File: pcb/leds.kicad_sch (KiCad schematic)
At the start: 55 parts

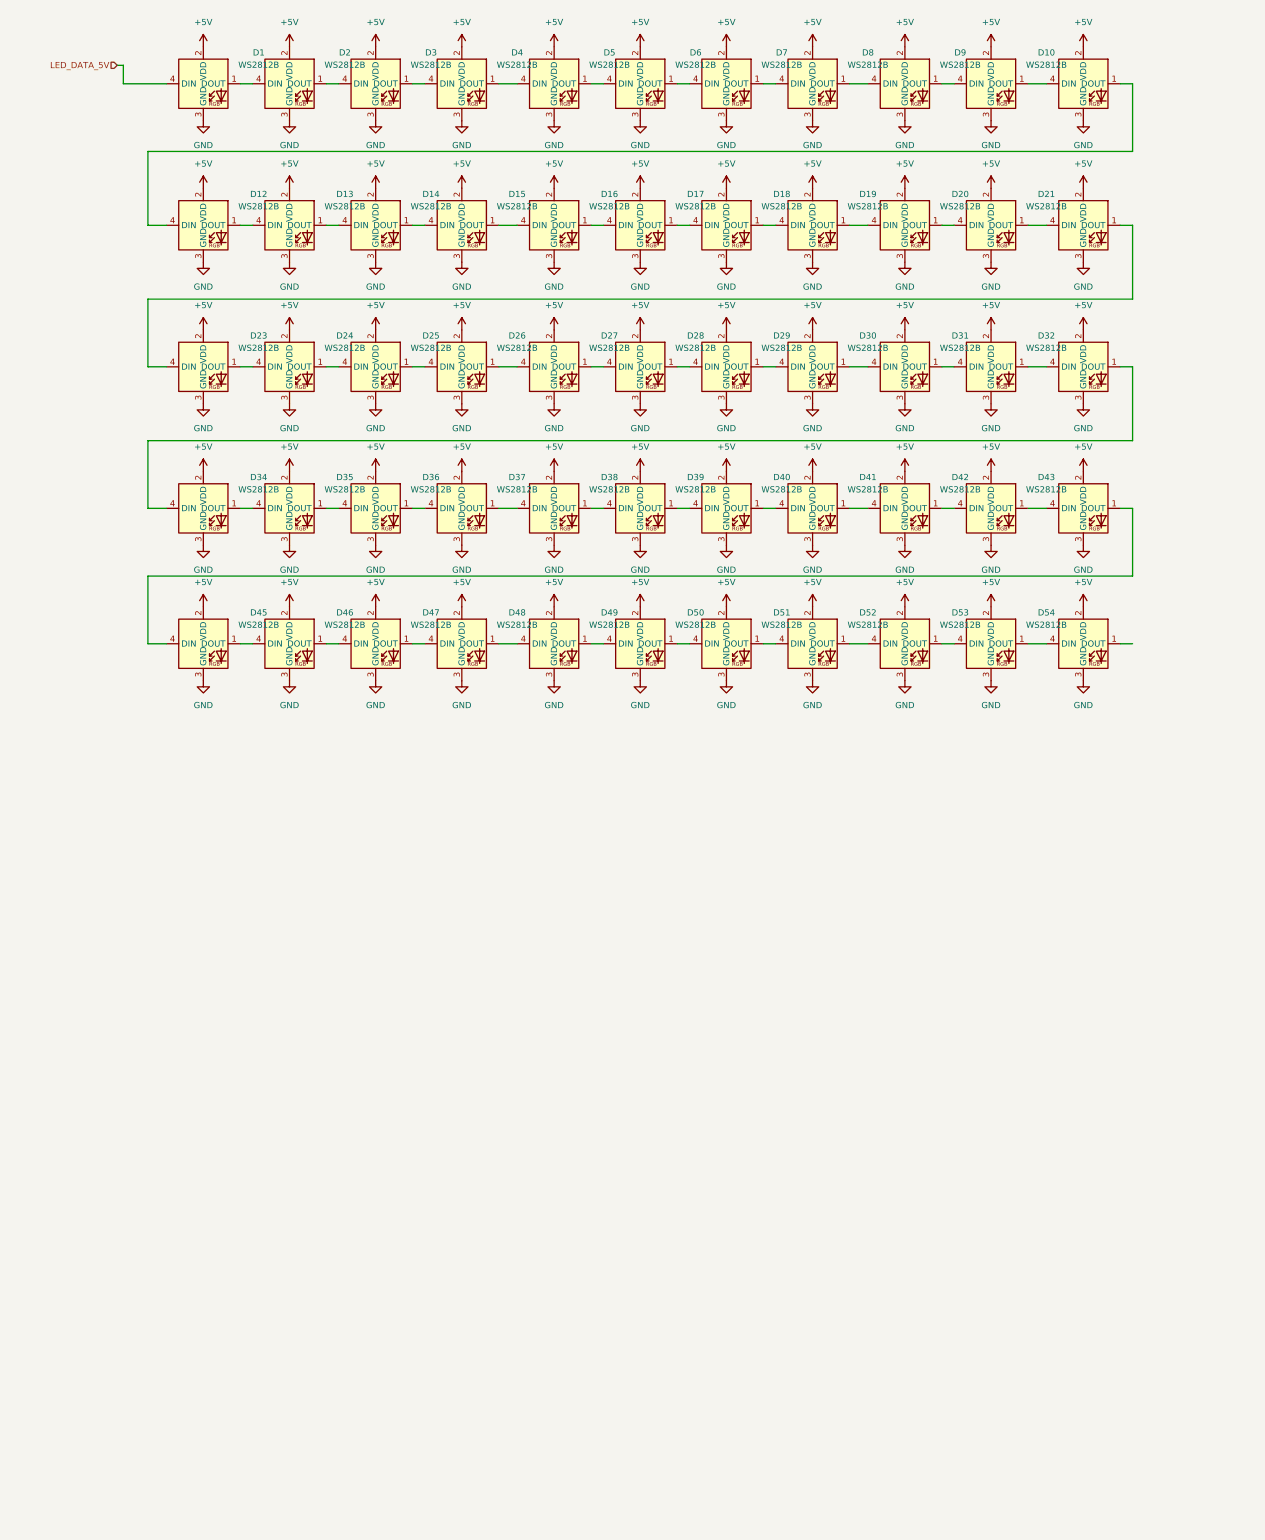
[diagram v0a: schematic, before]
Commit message: server updates and battling with kicad
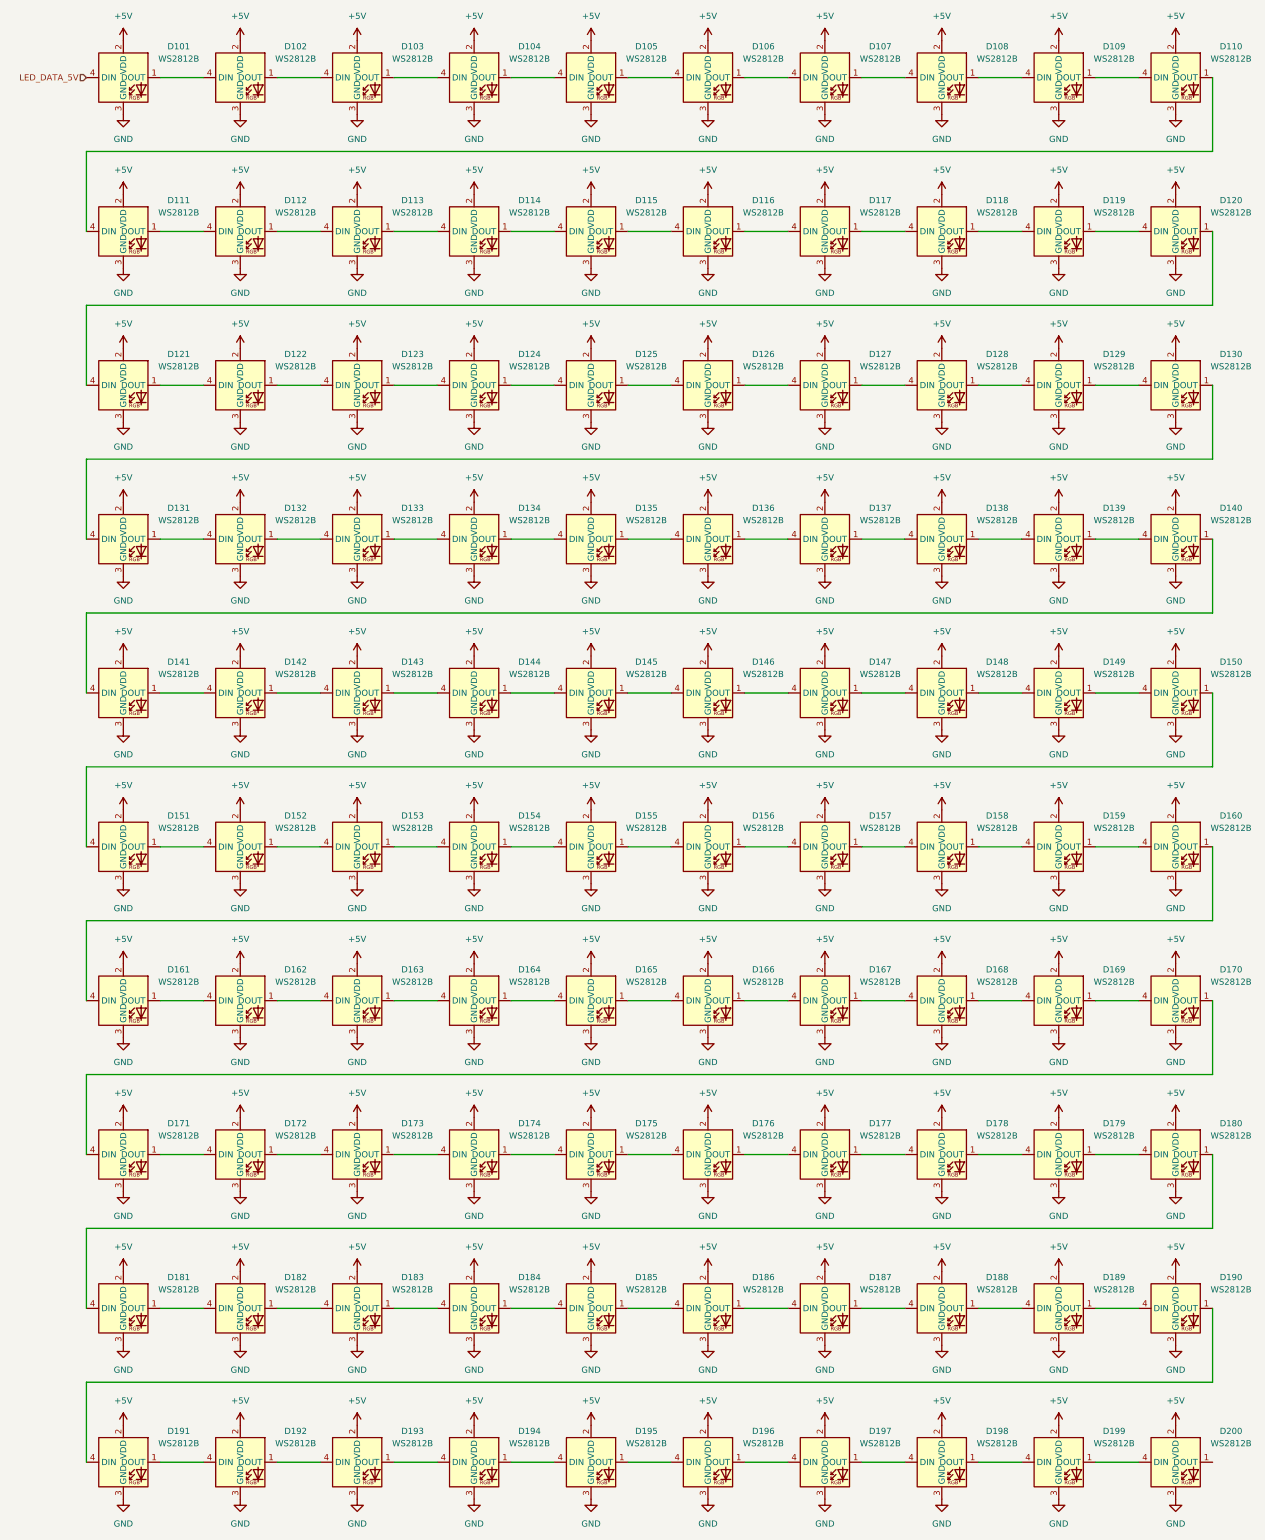
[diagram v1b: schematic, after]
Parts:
- removed D10, D11, D12, D13, D14, D15, D16, D17, D18, D19, D2, D20, D21, D22, D23, D24, D25, D26, D27, D28, D29, D3, D30, D31, D32, D33, D34, D35, D36, D37, D38, D39, D4, D40, D41, D42, D43, D44, D45, D46, D47, D48, D49, D5, D50, D51, D52, D53, D54, D55, D6, D7, D8, D9: WS2812B, PCM_JLCPCB:LED-SMD_4P-L1.6-W1.5_XL-1615RGBC-WS2812B, symbol PCM_JLCPCB-Extended:LED, WS2812B, 1615
- added D102, D103, D104, D105, D106, D107, D108, D109, D110, D111, D112, D113, D114, D115, D116, D117, D118, D119, D120, D121, D122, D123, D124, D125, D126, D127, D128, D129, D130, D131, D132, D133, D134, D135, D136, D137, D138, D139, D140, D141, D142, D143, D144, D145, D146, D147, D148, D149, D150, D151, D152, D153, D154, D155, D156, D157, D158, D159, D160, D161, D162, D163, D164, D165, D166, D167, D168, D169, D170, D171, D172, D173, D174, D175, D176, D177, D178, D179, D180, D181, D182, D183, D184, D185, D186, D187, D188, D189, D190, D191, D192, D193, D194, D195, D196, D197, D198, D199, D200: WS2812B, PCM_JLCPCB:LED-SMD_4P-L1.6-W1.5_XL-1615RGBC-WS2812B, symbol PCM_JLCPCB-Extended:LED, WS2812B, 1615
- renumbered D1 to D101
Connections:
- net +5V: now also D102.2 (VDD), D103.2 (VDD), D104.2 (VDD), D105.2 (VDD), D106.2 (VDD), D107.2 (VDD), D108.2 (VDD), D109.2 (VDD), D110.2 (VDD), D111.2 (VDD), D112.2 (VDD), D113.2 (VDD), D114.2 (VDD), D115.2 (VDD), D116.2 (VDD), D117.2 (VDD), D118.2 (VDD), D119.2 (VDD), D120.2 (VDD), D121.2 (VDD), D122.2 (VDD), D123.2 (VDD), D124.2 (VDD), D125.2 (VDD), D126.2 (VDD), D127.2 (VDD), D128.2 (VDD), D129.2 (VDD), D130.2 (VDD), D131.2 (VDD), D132.2 (VDD), D133.2 (VDD), D134.2 (VDD), D135.2 (VDD), D136.2 (VDD), D137.2 (VDD), D138.2 (VDD), D139.2 (VDD), D140.2 (VDD), D141.2 (VDD), D142.2 (VDD), D143.2 (VDD), D144.2 (VDD), D145.2 (VDD), D146.2 (VDD), D147.2 (VDD), D148.2 (VDD), D149.2 (VDD), D150.2 (VDD), D151.2 (VDD), D152.2 (VDD), D153.2 (VDD), D154.2 (VDD), D155.2 (VDD), D156.2 (VDD), D157.2 (VDD), D158.2 (VDD), D159.2 (VDD), D160.2 (VDD), D161.2 (VDD), D162.2 (VDD), D163.2 (VDD), D164.2 (VDD), D165.2 (VDD), D166.2 (VDD), D167.2 (VDD), D168.2 (VDD), D169.2 (VDD), D170.2 (VDD), D171.2 (VDD), D172.2 (VDD), D173.2 (VDD), D174.2 (VDD), D175.2 (VDD), D176.2 (VDD), D177.2 (VDD), D178.2 (VDD), D179.2 (VDD), D180.2 (VDD), D181.2 (VDD), D182.2 (VDD), D183.2 (VDD), D184.2 (VDD), D185.2 (VDD), D186.2 (VDD), D187.2 (VDD), D188.2 (VDD), D189.2 (VDD), D190.2 (VDD), D191.2 (VDD), D192.2 (VDD), D193.2 (VDD), D194.2 (VDD), D195.2 (VDD), D196.2 (VDD), D197.2 (VDD), D198.2 (VDD), D199.2 (VDD), D200.2 (VDD)
- net GND: now also D102.3 (GND), D103.3 (GND), D104.3 (GND), D105.3 (GND), D106.3 (GND), D107.3 (GND), D108.3 (GND), D109.3 (GND), D110.3 (GND), D111.3 (GND), D112.3 (GND), D113.3 (GND), D114.3 (GND), D115.3 (GND), D116.3 (GND), D117.3 (GND), D118.3 (GND), D119.3 (GND), D120.3 (GND), D121.3 (GND), D122.3 (GND), D123.3 (GND), D124.3 (GND), D125.3 (GND), D126.3 (GND), D127.3 (GND), D128.3 (GND), D129.3 (GND), D130.3 (GND), D131.3 (GND), D132.3 (GND), D133.3 (GND), D134.3 (GND), D135.3 (GND), D136.3 (GND), D137.3 (GND), D138.3 (GND), D139.3 (GND), D140.3 (GND), D141.3 (GND), D142.3 (GND), D143.3 (GND), D144.3 (GND), D145.3 (GND), D146.3 (GND), D147.3 (GND), D148.3 (GND), D149.3 (GND), D150.3 (GND), D151.3 (GND), D152.3 (GND), D153.3 (GND), D154.3 (GND), D155.3 (GND), D156.3 (GND), D157.3 (GND), D158.3 (GND), D159.3 (GND), D160.3 (GND), D161.3 (GND), D162.3 (GND), D163.3 (GND), D164.3 (GND), D165.3 (GND), D166.3 (GND), D167.3 (GND), D168.3 (GND), D169.3 (GND), D170.3 (GND), D171.3 (GND), D172.3 (GND), D173.3 (GND), D174.3 (GND), D175.3 (GND), D176.3 (GND), D177.3 (GND), D178.3 (GND), D179.3 (GND), D180.3 (GND), D181.3 (GND), D182.3 (GND), D183.3 (GND), D184.3 (GND), D185.3 (GND), D186.3 (GND), D187.3 (GND), D188.3 (GND), D189.3 (GND), D190.3 (GND), D191.3 (GND), D192.3 (GND), D193.3 (GND), D194.3 (GND), D195.3 (GND), D196.3 (GND), D197.3 (GND), D198.3 (GND), D199.3 (GND), D200.3 (GND)
- net at D101.1 (DOUT): now also D102.4 (DIN)
- new net: D134.1 (DOUT), D135.4 (DIN)
- new net: D133.1 (DOUT), D134.4 (DIN)
- new net: D187.1 (DOUT), D188.4 (DIN)
- new net: D186.1 (DOUT), D187.4 (DIN)
- new net: D160.1 (DOUT), D161.4 (DIN)
- new net: D159.1 (DOUT), D160.4 (DIN)
- new net: D149.1 (DOUT), D150.4 (DIN)
- new net: D148.1 (DOUT), D149.4 (DIN)
- new net: D180.1 (DOUT), D181.4 (DIN)
- new net: D179.1 (DOUT), D180.4 (DIN)
- new net: D116.1 (DOUT), D117.4 (DIN)
- new net: D115.1 (DOUT), D116.4 (DIN)
- new net: D195.1 (DOUT), D196.4 (DIN)
- new net: D194.1 (DOUT), D195.4 (DIN)
- new net: D141.1 (DOUT), D142.4 (DIN)
- new net: D140.1 (DOUT), D141.4 (DIN)
- new net: D163.1 (DOUT), D164.4 (DIN)
- new net: D162.1 (DOUT), D163.4 (DIN)
- new net: D193.1 (DOUT), D194.4 (DIN)
- new net: D192.1 (DOUT), D193.4 (DIN)
- new net: D183.1 (DOUT), D184.4 (DIN)
- new net: D182.1 (DOUT), D183.4 (DIN)
- new net: D161.1 (DOUT), D162.4 (DIN)
- new net: D171.1 (DOUT), D172.4 (DIN)
- new net: D170.1 (DOUT), D171.4 (DIN)
- new net: D185.1 (DOUT), D186.4 (DIN)
- new net: D132.1 (DOUT), D133.4 (DIN)
- new net: D165.1 (DOUT), D166.4 (DIN)
- new net: D164.1 (DOUT), D165.4 (DIN)
- new net: D156.1 (DOUT), D157.4 (DIN)
- new net: D155.1 (DOUT), D156.4 (DIN)
- new net: D181.1 (DOUT), D182.4 (DIN)
- new net: D113.1 (DOUT), D114.4 (DIN)
- new net: D112.1 (DOUT), D113.4 (DIN)
- new net: D138.1 (DOUT), D139.4 (DIN)
- new net: D137.1 (DOUT), D138.4 (DIN)
- new net: D168.1 (DOUT), D169.4 (DIN)
- new net: D167.1 (DOUT), D168.4 (DIN)
- new net: D197.1 (DOUT), D198.4 (DIN)
- new net: D196.1 (DOUT), D197.4 (DIN)
- new net: D188.1 (DOUT), D189.4 (DIN)
- new net: D199.1 (DOUT), D200.4 (DIN)
- new net: D126.1 (DOUT), D127.4 (DIN)
- new net: D125.1 (DOUT), D126.4 (DIN)
- new net: D106.1 (DOUT), D107.4 (DIN)
- new net: D105.1 (DOUT), D106.4 (DIN)
- new net: D108.1 (DOUT), D109.4 (DIN)
- new net: D107.1 (DOUT), D108.4 (DIN)
- new net: D169.1 (DOUT), D170.4 (DIN)
- new net: D109.1 (DOUT), D110.4 (DIN)
- new net: D103.1 (DOUT), D104.4 (DIN)
- new net: D102.1 (DOUT), D103.4 (DIN)
- new net: D198.1 (DOUT), D199.4 (DIN)
- new net: D111.1 (DOUT), D112.4 (DIN)
- new net: D110.1 (DOUT), D111.4 (DIN)
- new net: D118.1 (DOUT), D119.4 (DIN)
- new net: D117.1 (DOUT), D118.4 (DIN)
- new net: D130.1 (DOUT), D131.4 (DIN)
- new net: D129.1 (DOUT), D130.4 (DIN)
- new net: D178.1 (DOUT), D179.4 (DIN)
- new net: D114.1 (DOUT), D115.4 (DIN)
- new net: D158.1 (DOUT), D159.4 (DIN)
- new net: D157.1 (DOUT), D158.4 (DIN)
- new net: D144.1 (DOUT), D145.4 (DIN)
- new net: D143.1 (DOUT), D144.4 (DIN)
- new net: D189.1 (DOUT), D190.4 (DIN)
- new net: D147.1 (DOUT), D148.4 (DIN)
- new net: D146.1 (DOUT), D147.4 (DIN)
- new net: D151.1 (DOUT), D152.4 (DIN)
- new net: D150.1 (DOUT), D151.4 (DIN)
- new net: D190.1 (DOUT), D191.4 (DIN)
- new net: D119.1 (DOUT), D120.4 (DIN)
- new net: D124.1 (DOUT), D125.4 (DIN)
- new net: D122.1 (DOUT), D123.4 (DIN)
- new net: D121.1 (DOUT), D122.4 (DIN)
- new net: D174.1 (DOUT), D175.4 (DIN)
- new net: D173.1 (DOUT), D174.4 (DIN)
- new net: D184.1 (DOUT), D185.4 (DIN)
- new net: D172.1 (DOUT), D173.4 (DIN)
- new net: D142.1 (DOUT), D143.4 (DIN)
- new net: D123.1 (DOUT), D124.4 (DIN)
- new net: D128.1 (DOUT), D129.4 (DIN)
- new net: D175.1 (DOUT), D176.4 (DIN)
- new net: D120.1 (DOUT), D121.4 (DIN)
- new net: D154.1 (DOUT), D155.4 (DIN)
- new net: D153.1 (DOUT), D154.4 (DIN)
- new net: D145.1 (DOUT), D146.4 (DIN)
- new net: D166.1 (DOUT), D167.4 (DIN)
- new net: D135.1 (DOUT), D136.4 (DIN)
- new net: D152.1 (DOUT), D153.4 (DIN)
- new net: D131.1 (DOUT), D132.4 (DIN)
- new net: D104.1 (DOUT), D105.4 (DIN)
- new net: D177.1 (DOUT), D178.4 (DIN)
- new net: D139.1 (DOUT), D140.4 (DIN)
- new net: D191.1 (DOUT), D192.4 (DIN)
- new net: D136.1 (DOUT), D137.4 (DIN)
- new net: D176.1 (DOUT), D177.4 (DIN)
- new net: D127.1 (DOUT), D128.4 (DIN)
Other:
- moved on the sheet: D101
